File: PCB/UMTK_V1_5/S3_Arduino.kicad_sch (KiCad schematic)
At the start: 37 parts, among them SW1 Tac Switch, SW2 Tac Switch, SW3 Tac Switch, SW4 Tac Switch, SW5 Tac Switch, SW6 Tac Switch

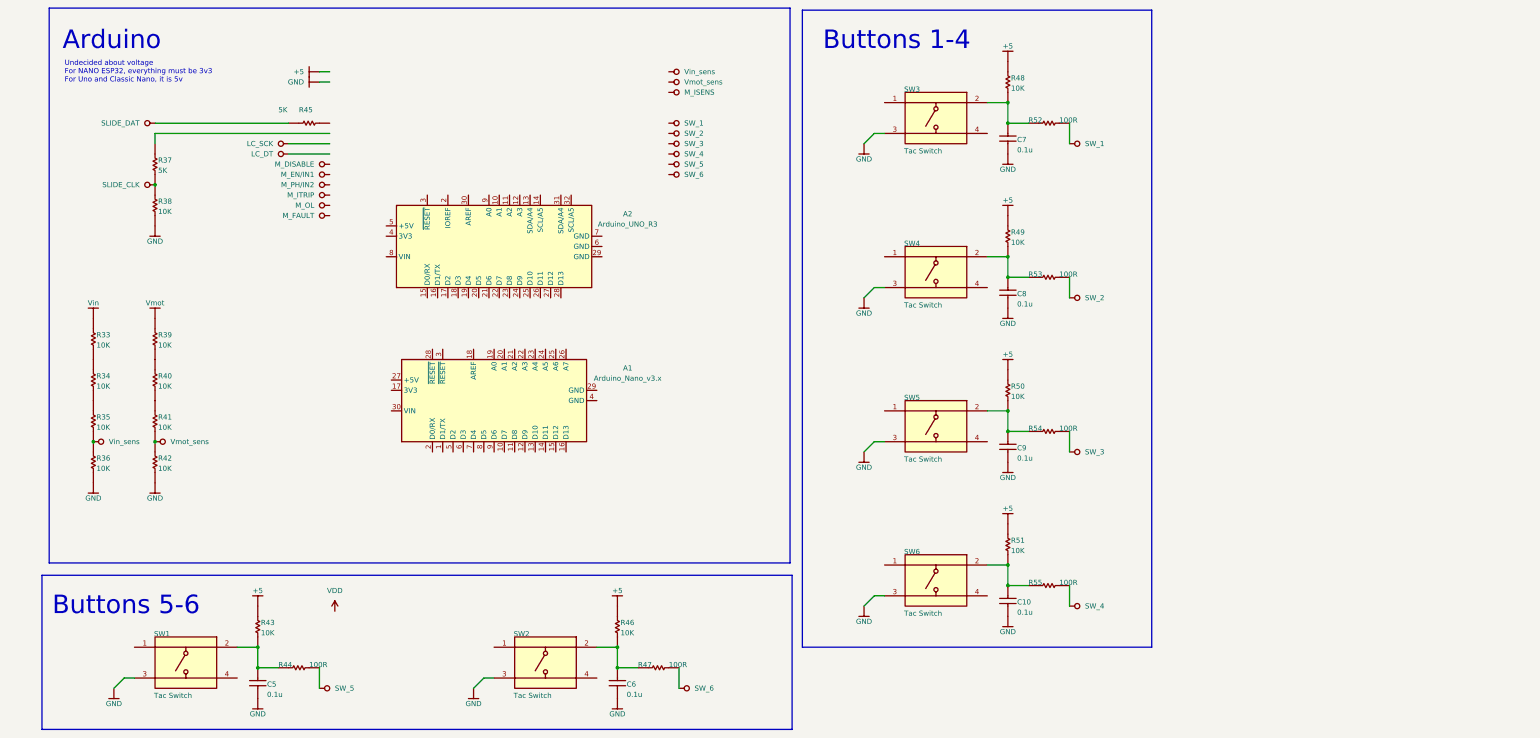
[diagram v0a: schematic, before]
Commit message: Updating Schematic
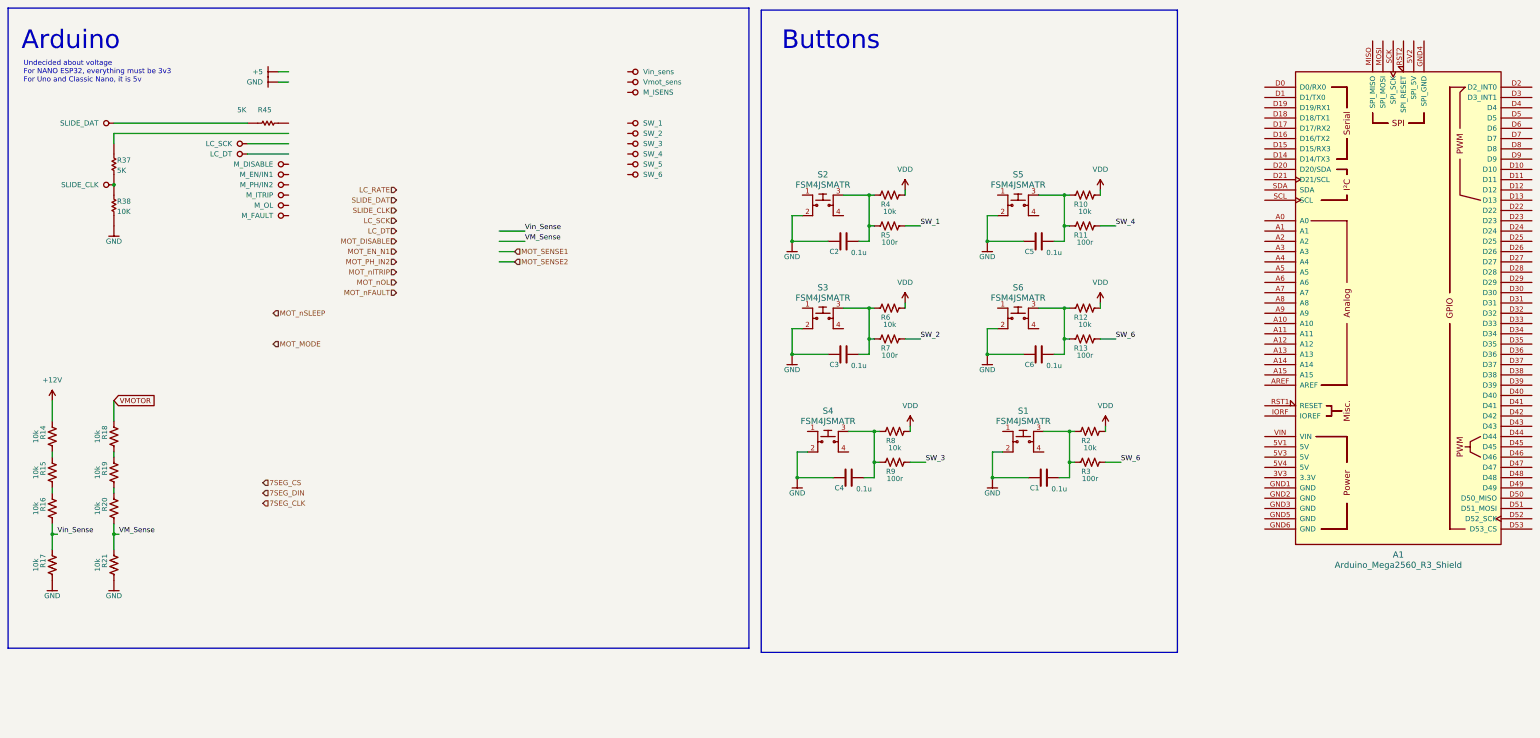
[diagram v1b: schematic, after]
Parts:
- removed A1: Arduino_Nano_v3.x, Module:Arduino_Nano, symbol MCU_Module:Arduino_Nano_v3.x
- removed A2: Arduino_UNO_R3, Module:Arduino_UNO_R3, symbol MCU_Module:Arduino_UNO_R3
- removed C10, C5, C6, C7, C8, C9: 0.1u, Ceramic Cap 5mm, symbol UMTK-altium-import:root_0_Cap
- removed R33, R34, R35, R36, R39, R40, R41, R42, R43, R46, R48, R49, R50, R51: Res1, AXIAL-0.3-3D, symbol UMTK-altium-import:root_3_Res1
- removed R44, R47, R52, R53, R54, R55: Res1, AXIAL-0.3-3D, symbol UMTK-altium-import:root_0_Res1
- removed SW1, SW2, SW3, SW4, SW5, SW6: Tac Switch, TacSwitch, symbol UMTK-altium-import:root_0_Tac Switch
- added A1: Arduino_Mega2560_R3_Shield, PCM_arduino-library:Arduino_Mega2560_R3_Shield, symbol arduino-library:Arduino_Mega2560_R3_Shield
- added C1, C2, C3, C4, C5, C6: 0.1u, symbol Device:C
- added R10, R12, R14, R15, R16, R17, R18, R19, R2, R20, R21, R4, R6, R8: 10k, symbol Device:R_US
- added R11, R13, R3, R5, R7, R9: 100r, symbol Device:R_US
- added S1, S2, S3, S4, S5, S6: FSM4JSMATR, digikey-footprints:Switch_Tactile_SMD_6x6mm, symbol dk_Tactile-Switches:FSM4JSMATR
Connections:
- net GND: now also C1.1, C2.1, C3.1, C4.1, C5.1, C6.1, R17.2, R21.2, S1.2, S2.2, S3.2, S4.2, S5.2, S6.2
- net SW_1: now also R5.2
- net SW_2: now also R7.2
- net SW_3: now also R9.2
- net SW_4: now also R11.2
- net SW_6: now also R13.2, R3.2
- net VDD: now also R10.2, R12.2, R2.2, R4.2, R6.2, R8.2
- new net: C1.2, R2.1, R3.1, S1.3
- new net: C4.2, R8.1, R9.1, S4.3
- new net: C5.2, R10.1, R11.1, S5.3
- new net: C6.2, R12.1, R13.1, S6.3
- new net: C3.2, R6.1, R7.1, S3.3
- new net: C2.2, R4.1, R5.1, S2.3
- new net: R14.2, R15.1
- new net: R15.2, R16.1
- new net: R18.2, R19.1
- new net: R19.2, R20.1
- new net +12V: R14.1
- new net VMOTOR: R18.1
- new net VM_Sense: R20.2, R21.1
- new net Vin_Sense: R16.2, R17.1
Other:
- note added: "Buttons"
- note removed: "Buttons 1-4"
- note removed: "Buttons 5-6"
- moved on the sheet: R37, R38, R45
